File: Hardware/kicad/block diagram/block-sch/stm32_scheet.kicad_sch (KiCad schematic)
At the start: 37 parts, among them J3 USB_A, J4 Conn_01x03, J5 Conn_02x02_Counter_Clockwise, Q2 BC817, SW1 NRST_BUTT, U16 CS43L21, U17 CAT24C256, U18 USBLC6-4SC6, U6 STM32L4Q5, Y1 Crystal

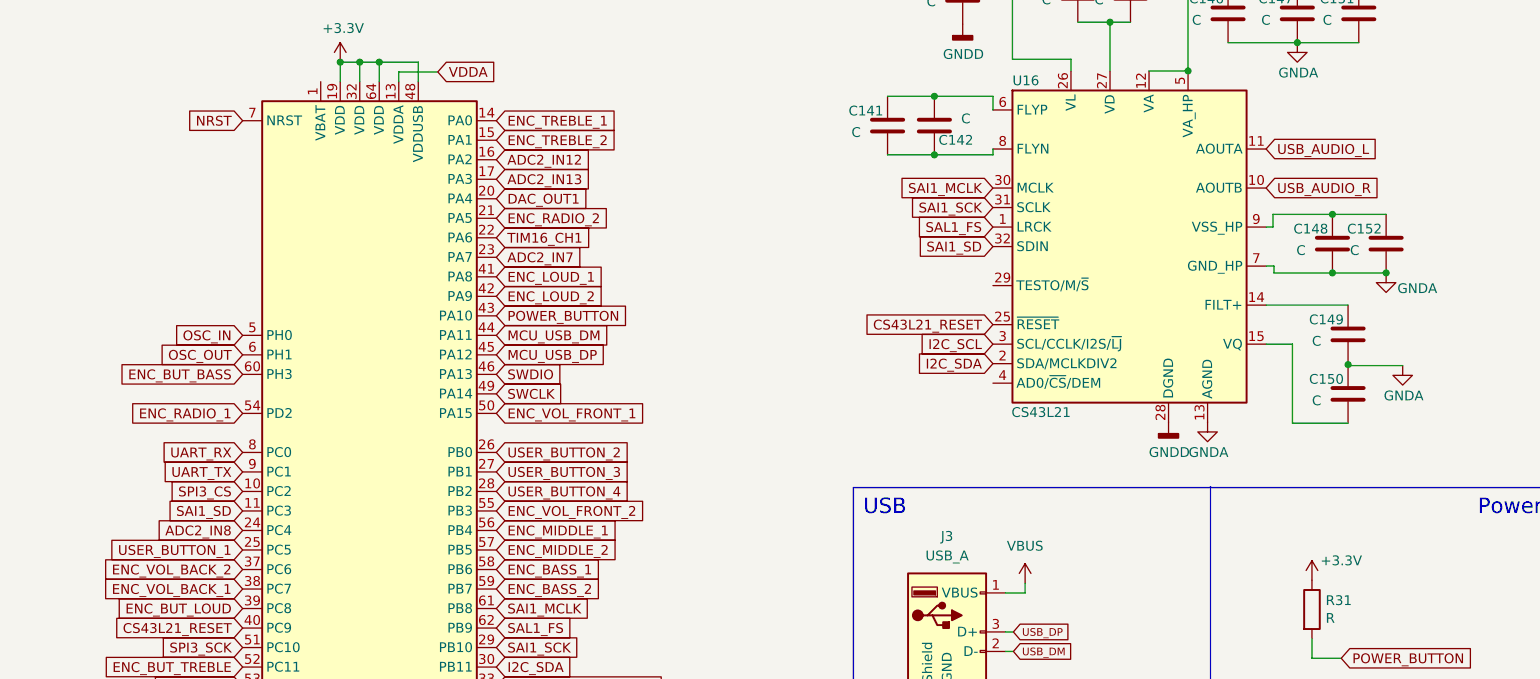
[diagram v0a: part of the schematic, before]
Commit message: new
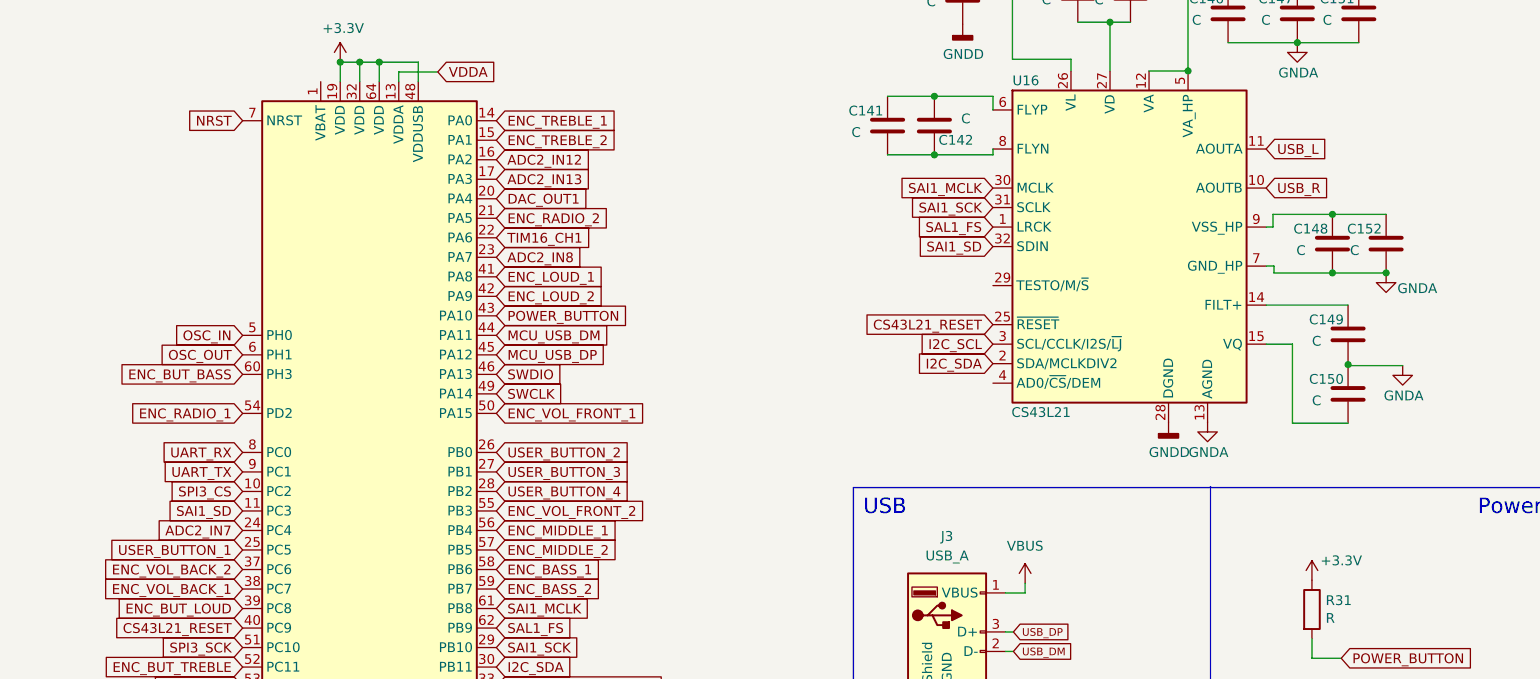
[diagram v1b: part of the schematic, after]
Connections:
- net ADC2_IN7: now also U6.24 (PC4); no longer U6.23 (PA7)
- net ADC2_IN8: now also U6.23 (PA7); no longer U6.24 (PC4)
- net USB_AUDIO_L renamed USB_L
- net USB_AUDIO_R renamed USB_R
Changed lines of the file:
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@@
     )
   )
-  (global_label "USB_AUDIO_R" (shape input) (at 184.531 91.821 0) (fields_autoplaced)
+  (global_label "USB_R" (shape input) (at 184.531 91.821 0) (fields_autoplaced)
     (effects (font (size 1.27 1.27)) (justify left))
-    (property "Intersheet References" "${INTERSHEET_REFS}" (id 0) (at 199.4947 91.7416 0)
+    (property "Intersheet References" "${INTERSHEET_REFS}" (id 0) (at 192.9028 91.7416 0)
       (effects (font (size 1.27 1.27)) (justify left) hide)
     )
@@
     )
   )
-  (global_label "ADC2_IN7" (shape input) (at 84.328 100.838 0) (fields_autoplaced)
-    (effects (font (size 1.27 1.27)) (justify left))
-    (property "Intersheet References" "${INTERSHEET_REFS}" (id 0) (at 11.938 30.988 0)
+  (global_label "ADC2_IN7" (shape input) (at 51.308 136.398 180) (fields_autoplaced)
+    (effects (font (size 1.27 1.27)) (justify right))
+    (property "Intersheet References" "${INTERSHEET_REFS}" (id 0) (at 123.698 206.248 0)
       (effects (font (size 1.27 1.27)) hide)
     )
   )
-  (global_label "ADC2_IN8" (shape input) (at 51.308 136.398 180) (fields_autoplaced)
-    (effects (font (size 1.27 1.27)) (justify right))
-    (property "Intersheet References" "${INTERSHEET_REFS}" (id 0) (at 123.698 208.788 0)
+  (global_label "ADC2_IN8" (shape input) (at 84.328 100.838 0) (fields_autoplaced)
+    (effects (font (size 1.27 1.27)) (justify left))
+    (property "Intersheet References" "${INTERSHEET_REFS}" (id 0) (at 11.938 28.448 0)
       (effects (font (size 1.27 1.27)) hide)
     )
   )
-  (global_label "USB_AUDIO_L" (shape input) (at 184.531 86.741 0) (fields_autoplaced)
+  (global_label "USB_L" (shape input) (at 184.531 86.741 0) (fields_autoplaced)
     (effects (font (size 1.27 1.27)) (justify left))
-    (property "Intersheet References" "${INTERSHEET_REFS}" (id 0) (at 199.2528 86.6616 0)
+    (property "Intersheet References" "${INTERSHEET_REFS}" (id 0) (at 192.6609 86.6616 0)
       (effects (font (size 1.27 1.27)) (justify left) hide)
     )
